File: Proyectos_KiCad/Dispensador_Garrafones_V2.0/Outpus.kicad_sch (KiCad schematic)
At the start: 43 parts, among them J10 LOAD, J5 LOAD, J6 LOAD, J7 LOAD, J8 LOAD, J9 LOAD, Q1 TIP122, Q2 BT136-800, Q3 BT136-800, Q4 BT136-800, Q5 BT136-800, Q7 BTA41-600B, U3 PC817, U4 MOC3021M, U5 MOC3021M, U6 MOC3021M, U7 MOC3021M

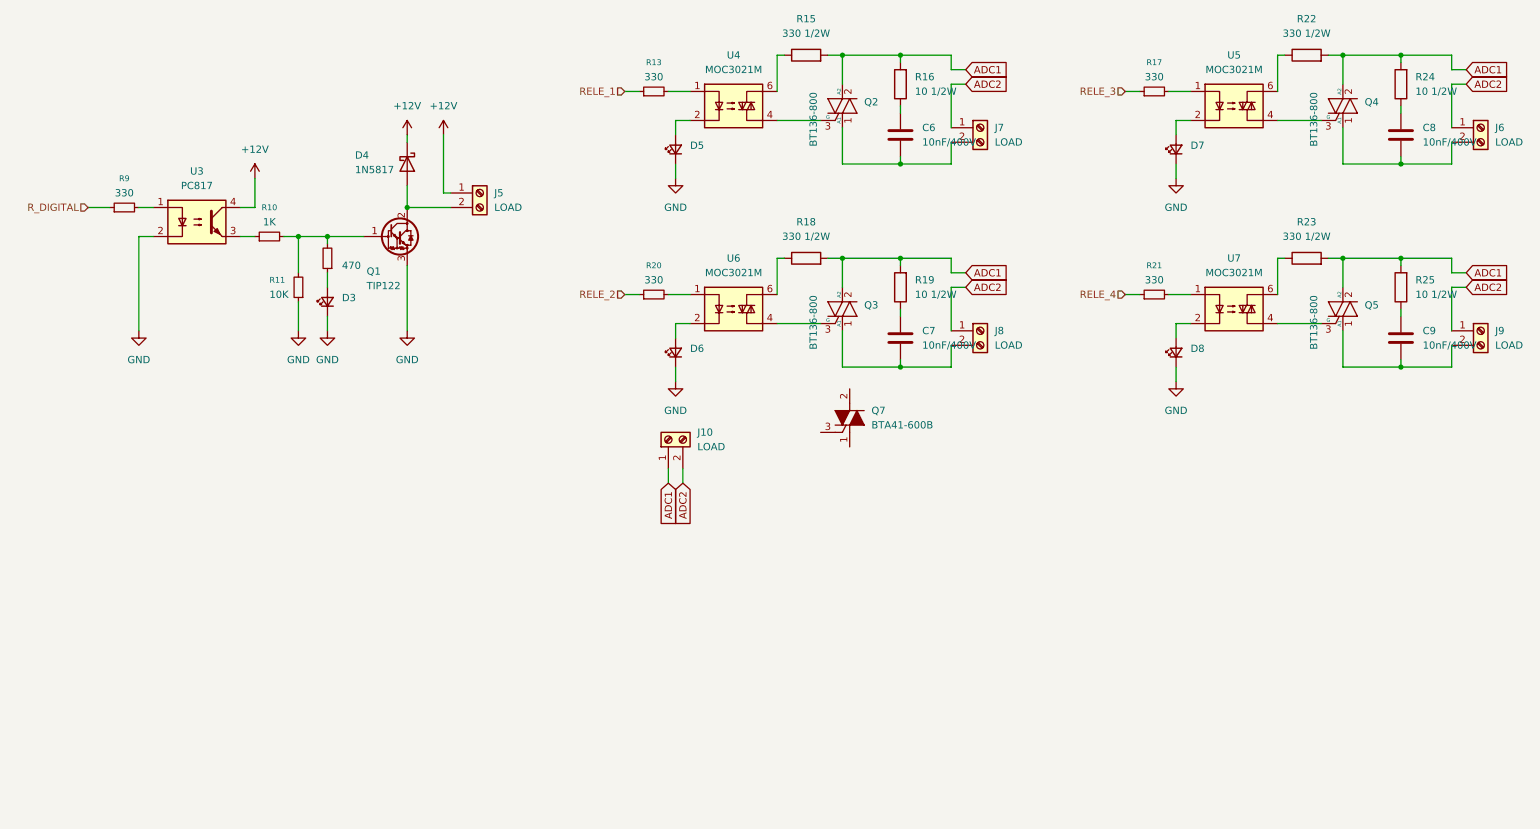
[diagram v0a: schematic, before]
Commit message: Backup antes de reinstalacion del SO: proyectos y librerias KiCad
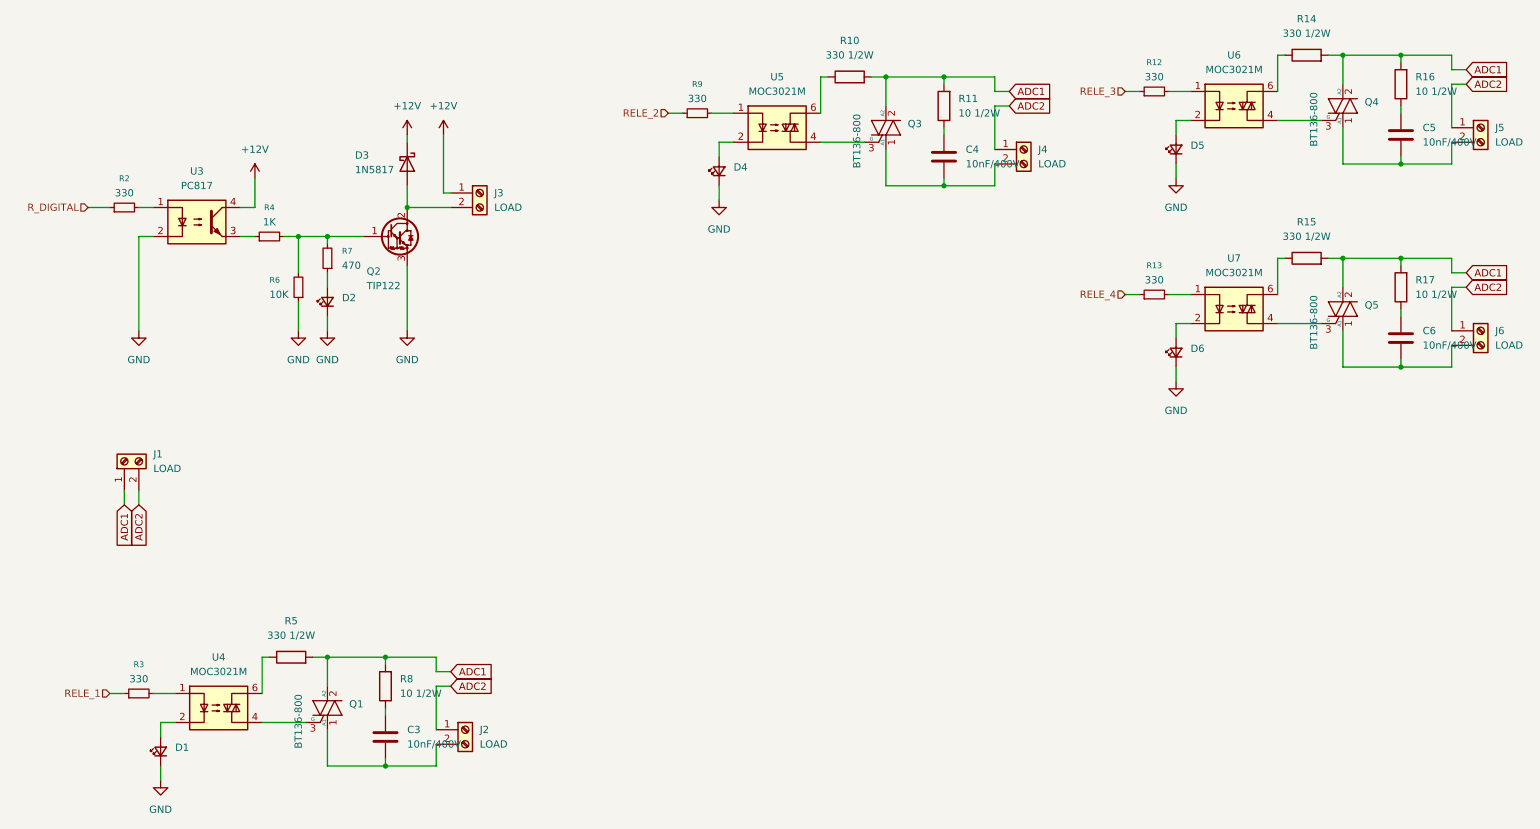
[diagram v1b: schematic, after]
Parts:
- removed Q7: BTA41-600B, PCM_Package_TO_SOT_THT_AKL:TO-218-3_Vertical_AAG, symbol PCM_Triac_AKL:BTA41-600B
- renumbered C6 to C3, C7 to C4, C8 to C5, C9 to C6, D5 to D1, D3 to D2, D4 to D3, D6 to D4, D7 to D5, D8 to D6, J10 to J1, J7 to J2, J5 to J3, J8 to J4, J6 to J5, J9 to J6, Q2 to Q1, Q1 to Q2, R18 to R10, R19 to R11, R17 to R12, R21 to R13, R22 to R14, R23 to R15, R24 to R16, R25 to R17, R9 to R2, R13 to R3, R10 to R4, R15 to R5, R11 to R6, R12 to R7, R16 to R8, R20 to R9, U6 to U5, U5 to U6
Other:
- moved on the sheet: C3, C4, D1, D4, J1, J2, J4, Q1, Q3, R10, R11, R3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
